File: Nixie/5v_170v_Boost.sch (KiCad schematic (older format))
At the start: 34 parts, among them Q3 MMBTA42, Q4 FDS2672CT, U9 UCC3803

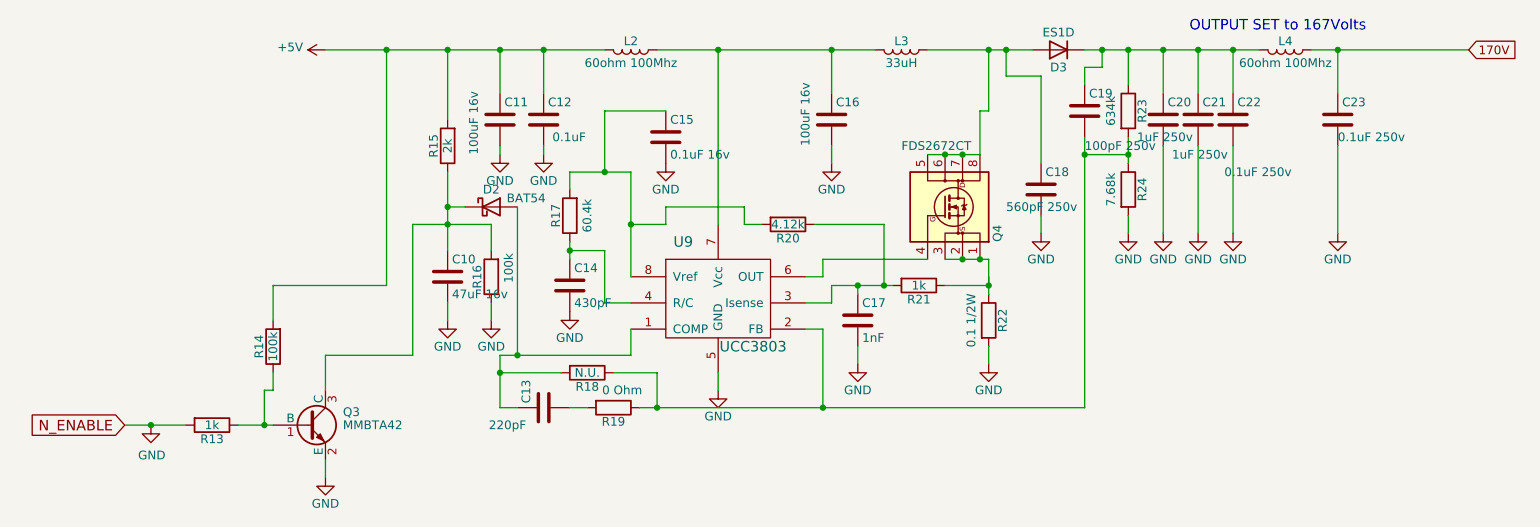
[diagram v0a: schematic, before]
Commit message: Kleinere Anpassungen
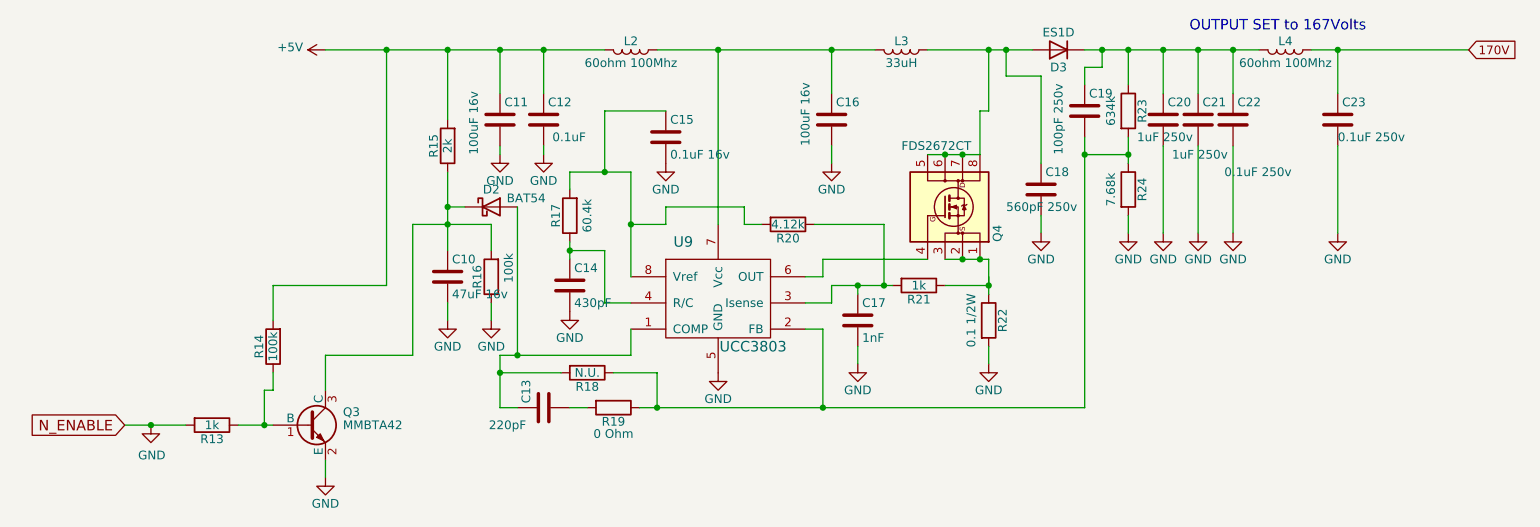
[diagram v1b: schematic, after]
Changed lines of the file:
@@
 L power:GND #PWR039
 U 1 1 58854BC1
-P 4600 4000
-F 0 "#PWR039" H 4600 3750 50  0001 C CNN
-F 1 "GND" H 4600 3850 50  0000 C CNN
-F 2 "" H 4600 4000 50  0000 C CNN
-F 3 "" H 4600 4000 50  0000 C CNN
-	1    4600 4000
+P 4600 3900
+F 0 "#PWR039" H 4600 3650 50  0001 C CNN
+F 1 "GND" H 4600 3750 50  0000 C CNN
+F 2 "" H 4600 3900 50  0000 C CNN
+F 3 "" H 4600 3900 50  0000 C CNN
+	1    4600 3900
 	1    0    0    -1
 $EndComp
@@
 P 4000 4100
 F 0 "R19" V 4080 4100 50  0000 C CNN
-F 1 "0 Ohm" V 3900 4150 50  0000 C CNN
+F 1 "0 Ohm" V 4150 4100 50  0000 C CNN
 F 2 "Resistors_SMD:R_0805" V 3930 4100 50  0001 C CNN
 F 3 "" H 4000 4100 50  0000 C CNN
@@
 P 6700 2400
 F 0 "C19" H 6725 2500 50  0000 L CNN
-F 1 "100pF 250v" H 6700 2200 50  0000 L CNN
+F 1 "100pF 250v" V 6550 2150 50  0000 L CNN
 F 2 "Capacitors_SMD:C_0805" H 6738 2250 50  0001 C CNN
 F 3 "https://www.digikey.com/products/en/capacitors/ceramic-capacitors/60?k=C0805C101JAGAC7800&k=&pkeyword=C0805C101JAGAC7800&pv7=2&quantity=0&ColumnSort=0&page=1&pageSize=25" H 6700 2400 50  0001 C CNN
@@
 $EndComp
 Wire Wire Line
-	4600 4000 4600 3900
-Wire Wire Line
 	4250 2050 4600 2050
